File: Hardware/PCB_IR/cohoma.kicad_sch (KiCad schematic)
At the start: 11 parts, among them J2 Conn_01x03, U1 MCP2120-I/P, U2 TSOP75338WTT, Y1 ABLS-7.3728MHz-20-B-3-H-T

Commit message: pcb sans erreurs (mais avec track à 0.3)
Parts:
- C1, C2, C3: footprint Capacitor_SMD:C_0201_0603Metric_Pad0.64x0.40mm_HandSolder -> Capacitor_SMD:C_0603_1608Metric_Pad1.08x0.95mm_HandSolder
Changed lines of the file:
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@@
       (effects (font (size 1.27 1.27)) (justify left))
     )
-    (property "Footprint" "Capacitor_SMD:C_0201_0603Metric_Pad0.64x0.40mm_HandSolder" (at 229.5652 59.69 0)
+    (property "Footprint" "Capacitor_SMD:C_0603_1608Metric_Pad1.08x0.95mm_HandSolder" (at 229.5652 59.69 0)
       (effects (font (size 1.27 1.27)) hide)
     )
@@
       (effects (font (size 1.27 1.27)) (justify left))
     )
-    (property "Footprint" "Capacitor_SMD:C_0201_0603Metric_Pad0.64x0.40mm_HandSolder" (at 210.5152 142.24 0)
+    (property "Footprint" "Capacitor_SMD:C_0603_1608Metric_Pad1.08x0.95mm_HandSolder" (at 210.5152 142.24 0)
       (effects (font (size 1.27 1.27)) hide)
     )
@@
       (effects (font (size 1.27 1.27)) (justify left))
     )
-    (property "Footprint" "Capacitor_SMD:C_0201_0603Metric_Pad0.64x0.40mm_HandSolder" (at 258.7752 60.96 0)
+    (property "Footprint" "Capacitor_SMD:C_0603_1608Metric_Pad1.08x0.95mm_HandSolder" (at 258.7752 60.96 0)
       (effects (font (size 1.27 1.27)) hide)
     )

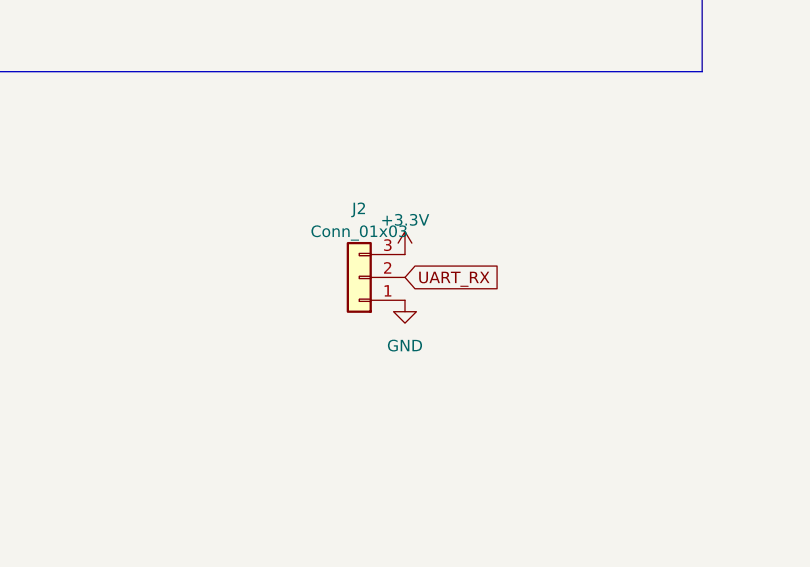
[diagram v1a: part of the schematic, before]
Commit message: final
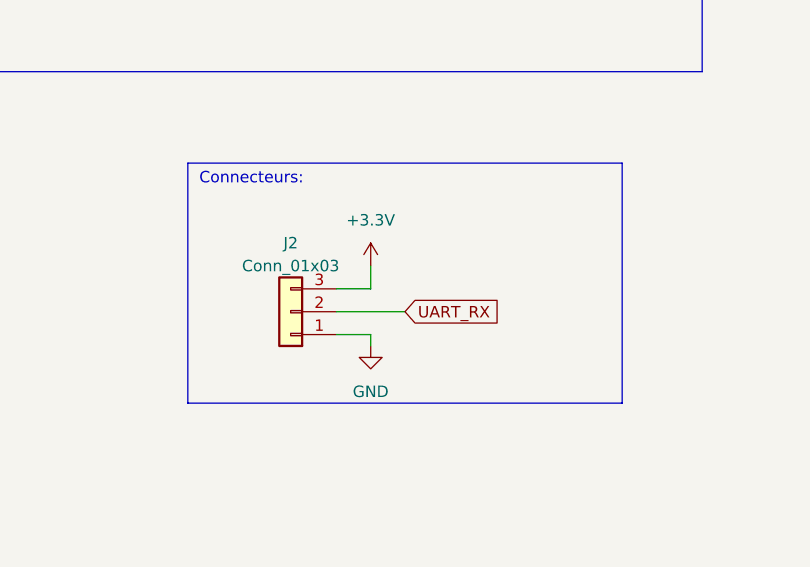
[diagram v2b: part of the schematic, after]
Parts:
- Y1: footprint Crystal:Crystal_SMD_EuroQuartz_MQ-4Pin_7.0x5.0mm -> Crystal:Crystal_SMD_7050-2Pin_7.0x5.0mm
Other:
- note added: "Connecteurs:"
- moved on the sheet: J2
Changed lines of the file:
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@@
+    (stroke (width 0) (type default))
+  )
+  (wire (pts (xy 68.58 132.08) (xy 72.39 132.08))
     (stroke (width 0) (type default))
   )
@@
     (stroke (width 0) (type default))
   )
+  (wire (pts (xy 68.58 129.54) (xy 76.2 129.54))
+    (stroke (width 0) (type default))
+  )
   (polyline (pts (xy 246.38 116.84) (xy 246.38 160.02))
     (stroke (width 0) (type default))
@@
     (stroke (width 0) (type default))
   )
+  (wire (pts (xy 72.39 132.08) (xy 72.39 133.35))
+    (stroke (width 0) (type default))
+  )
   (polyline (pts (xy 205.74 17.78) (xy 205.74 73.66))
     (stroke (width 0) (type default))
@@
     (stroke (width 0) (type default))
   )
+  (wire (pts (xy 68.58 127) (xy 72.39 127))
+    (stroke (width 0) (type default))
+  )
   (wire (pts (xy 196.85 128.27) (xy 207.01 128.27))
     (stroke (width 0) (type default))
@@
     (stroke (width 0) (type default))
   )
+  (wire (pts (xy 72.39 127) (xy 72.39 124.46))
+    (stroke (width 0) (type default))
+  )
+  (rectangle (start 52.07 113.03) (end 100.33 139.7)
+    (stroke (width 0) (type default))
+    (fill (type none))
+  )
   (text "Encodeur/décodeur" (at 17.78 22.86 0)
+    (effects (font (size 1.27 1.27)) (justify left bottom))
+  )
+  (text "Connecteurs:\n" (at 53.34 115.57 0)
     (effects (font (size 1.27 1.27)) (justify left bottom))
   )
@@
     )
   )
-  (global_label "UART_RX" (shape input) (at 76.2 125.73 0) (fields_autoplaced)
+  (global_label "UART_RX" (shape input) (at 76.2 129.54 0) (fields_autoplaced)
     (effects (font (size 1.27 1.27)) (justify left))
-    (property "Intersheetrefs" "${INTERSHEET_REFS}" (at 87.2096 125.73 0)
+    (property "Intersheetrefs" "${INTERSHEET_REFS}" (at 87.2096 129.54 0)
       (effects (font (size 1.27 1.27)) (justify left) hide)
     )
@@
       (effects (font (size 1.27 1.27)))
     )
-    (property "Footprint" "Crystal:Crystal_SMD_EuroQuartz_MQ-4Pin_7.0x5.0mm" (at 240.03 45.72 0)
+    (property "Footprint" "Crystal:Crystal_SMD_7050-2Pin_7.0x5.0mm" (at 240.03 45.72 0)
       (effects (font (size 1.27 1.27)) (justify bottom) hide)
     )
@@
     )
   )
-  (symbol (lib_id "power:+3.3V") (at 76.2 123.19 0) (unit 1)
-    (in_bom yes) (on_board yes) (dnp no) (fields_autoplaced)
-    (property "Reference" "#PWR09" (at 76.2 127 0)
-      (effects (font (size 1.27 1.27)) hide)
-    )
-    (property "Value" "+3.3V" (at 76.2 119.38 0)
-      (effects (font (size 1.27 1.27)))
-    )
-    (property "Footprint" "" (at 76.2 123.19 0)
-      (effects (font (size 1.27 1.27)) hide)
-    )
-    (property "Datasheet" "" (at 76.2 123.19 0)
+  (symbol (lib_id "power:+3.3V") (at 72.39 124.46 0) (unit 1)
+    (in_bom yes) (on_board yes) (dnp no)
+    (property "Reference" "#PWR09" (at 72.39 128.27 0)
+      (effects (font (size 1.27 1.27)) hide)
+    )
+    (property "Value" "+3.3V" (at 72.39 119.38 0)
+      (effects (font (size 1.27 1.27)))
+    )
+    (property "Footprint" "" (at 72.39 124.46 0)
+      (effects (font (size 1.27 1.27)) hide)
+    )
+    (property "Datasheet" "" (at 72.39 124.46 0)
       (effects (font (size 1.27 1.27)) hide)
     )
@@
     )
   )
-  (symbol (lib_id "power:GND") (at 76.2 128.27 0) (unit 1)
-    (in_bom yes) (on_board yes) (dnp no) (fields_autoplaced)
-    (property "Reference" "#PWR010" (at 76.2 134.62 0)
-      (effects (font (size 1.27 1.27)) hide)
-    )
-    (property "Value" "GND" (at 76.2 133.35 0)
-      (effects (font (size 1.27 1.27)))
-    )
-    (property "Footprint" "" (at 76.2 128.27 0)
-      (effects (font (size 1.27 1.27)) hide)
-    )
-    (property "Datasheet" "" (at 76.2 128.27 0)
+  (symbol (lib_id "power:GND") (at 72.39 133.35 0) (unit 1)
+    (in_bom yes) (on_board yes) (dnp no) (fields_autoplaced)
+    (property "Reference" "#PWR010" (at 72.39 139.7 0)
+      (effects (font (size 1.27 1.27)) hide)
+    )
+    (property "Value" "GND" (at 72.39 138.43 0)
+      (effects (font (size 1.27 1.27)))
+    )
+    (property "Footprint" "" (at 72.39 133.35 0)
+      (effects (font (size 1.27 1.27)) hide)
+    )
+    (property "Datasheet" "" (at 72.39 133.35 0)
       (effects (font (size 1.27 1.27)) hide)
     )
@@
     )
   )
-  (symbol (lib_id "Connector_Generic:Conn_01x03") (at 71.12 125.73 180) (unit 1)
-    (in_bom yes) (on_board yes) (dnp no) (fields_autoplaced)
-    (property "Reference" "J2" (at 71.12 118.11 0)
-      (effects (font (size 1.27 1.27)))
-    )
-    (property "Value" "Conn_01x03" (at 71.12 120.65 0)
-      (effects (font (size 1.27 1.27)))
-    )
-    (property "Footprint" "Connector_PinHeader_1.27mm:PinHeader_1x03_P1.27mm_Horizontal" (at 71.12 125.73 0)
-      (effects (font (size 1.27 1.27)) hide)
-    )
-    (property "Datasheet" "~" (at 71.12 125.73 0)
-      (effects (font (size 1.27 1.27)) hide)
-    )
+  (symbol (lib_id "Connector_Generic:Conn_01x03") (at 63.5 129.54 180) (unit 1)
+    (in_bom yes) (on_board yes) (dnp no) (fields_autoplaced)
+    (property "Reference" "J2" (at 63.5 121.92 0)
+      (effects (font (size 1.27 1.27)))
+    )
+    (property "Value" "Conn_01x03" (at 63.5 124.46 0)
+      (effects (font (size 1.27 1.27)))
+    )
+    (property "Footprint" "Connector_PinHeader_1.27mm:PinHeader_1x03_P1.27mm_Horizontal" (at 63.5 129.54 0)
+      (effects (font (size 1.27 1.27)) hide)
+    )
+    (property "Datasheet" "~" (at 63.5 129.54 0)
+      (effects (font (size 1.27 1.27)) hide)
+    )
